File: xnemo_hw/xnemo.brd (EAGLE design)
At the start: 38.6 x 29.8 mm, 34 parts, among them J1 MICRO_USB_B_RECEPT, J2 DM3D_MICRO_SD, J3 HEADER_2X5_0.05_SMD, J4 HEADER_2X5_0.05_THRU, J5 HEADER_2X5_0.05_THRU, U1 LTC3559, U2 L3GD20, U3 STM32F405RG, U5 HMC5883L, U6 ADXL345, X1 TXC_7A_XTAL

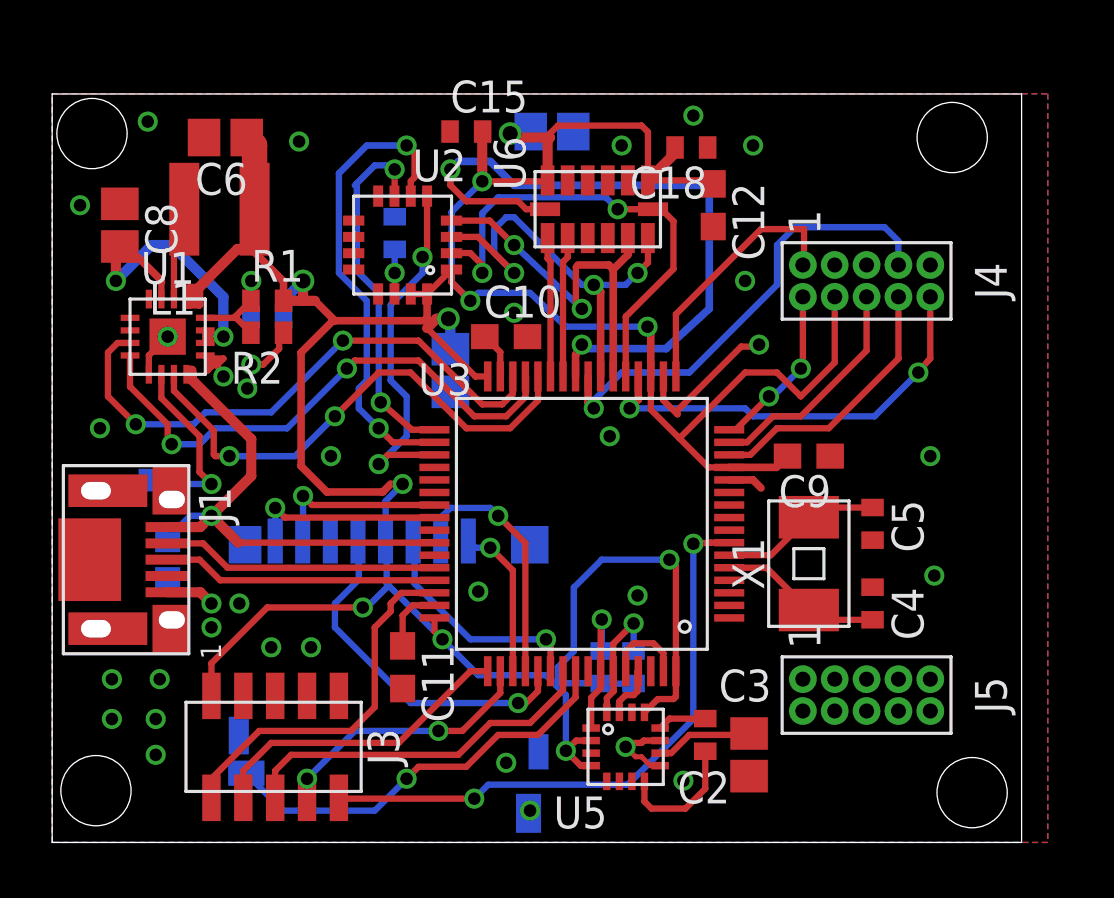
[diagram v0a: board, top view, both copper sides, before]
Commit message: r1 submitted
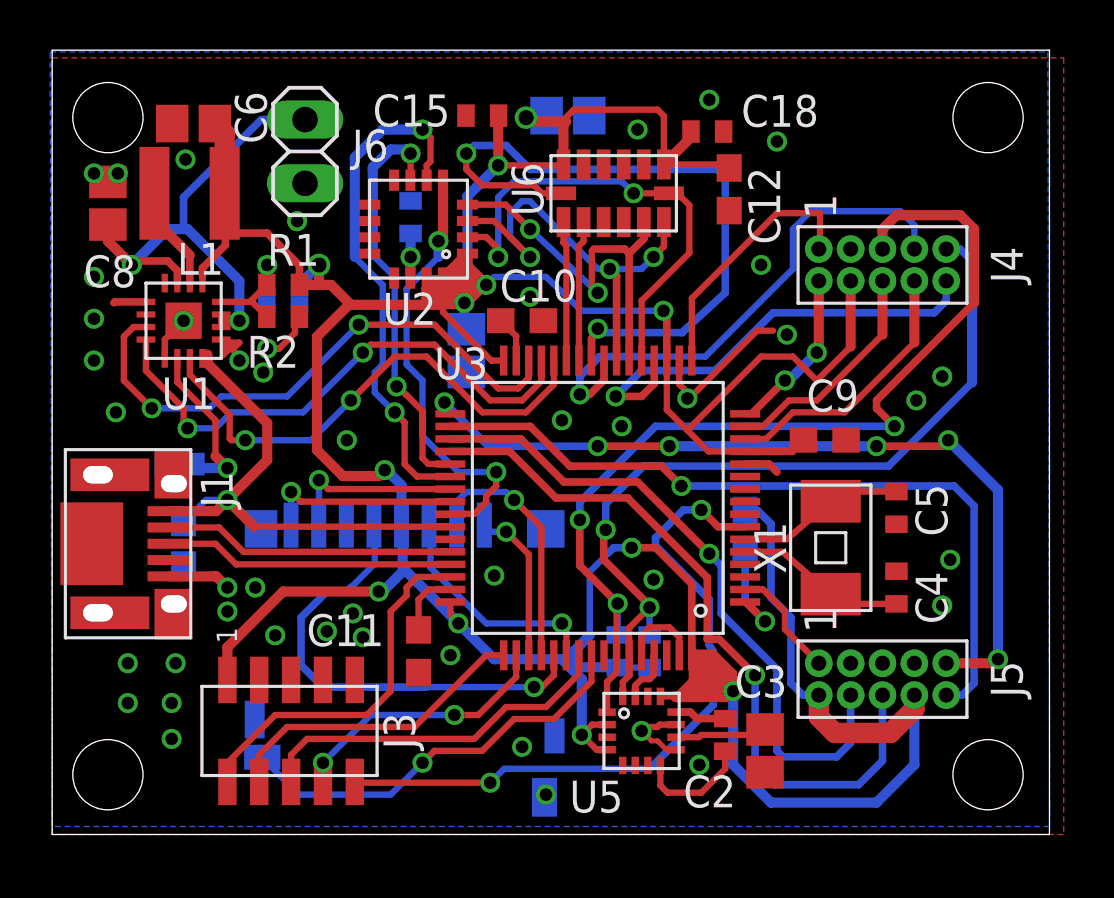
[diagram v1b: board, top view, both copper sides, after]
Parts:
- added C13: 2.2u, resistor:C0603
- added J6: (no value), pinhead:1X02
- moved C6 1.39 mm to (5.64, 28.3)
- moved L1 1.35 mm to (5.48, 25.6)
- moved C4 1.14 mm to (33.7, 9.84)
- moved C5 1.14 mm to (33.7, 13.0)
- moved X1 1.08 mm to (31.0, 11.4)
- moved C16 1.02 mm to (16.5, 19.3)
- moved C8 0.99 mm to (2.22, 25.2)
- moved J4 0.90 mm to (33.1, 22.7)
- moved J5 0.90 mm to (33.1, 6.19)
- moved C10 0.90 mm to (18.7, 20.5)
- moved C12 0.90 mm to (27.0, 25.7)
- moved C17 0.90 mm to (20.6, 28.7)
- moved U5 0.90 mm to (23.5, 4.13)
- moved C14 0.90 mm to (9.21, 21.3)
- moved J2 0.90 mm to (13.3, 6.35)
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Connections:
- removed net N$1: J5.P$4
- removed net N$16: J5.P$7
- removed net N$17: J5.P$5
- removed net N$2: J5.P$2
- removed net N$3: J5.P$3
- removed net N$4: J5.P$1
- removed net N$5: J5.P$6
- removed net N$6: J5.P$8
- removed net N$7: J4.P$9
- removed net N$8: J5.P$10
- removed net N$9: J5.P$9
- new net PA10: U3.P$43
- new net PB12: J5.P$9, U3.P$33
- new net PB13: J5.P$10, U3.P$34
- new net PB14: J5.P$4, U3.P$35
- new net PB15: J5.P$6, U3.P$36
- new net PC13: J5.P$1, U3.P$2
- new net UC_VBAT: C13.2, U3.P$1
- net 3V3: now also C13.1, J5.P$2, J5.P$8
- net GND: now also J5.P$3, J5.P$5, J5.P$7, J6.1
- net GYR_DRDY: now also U3.P$38; no longer U3.P$34
- net GYR_INT1: now also U3.P$37; no longer U3.P$33
- net I2C_SCL: now also J4.P$5
- net I2C_SDA: now also J4.P$9
- net PA1: no longer J4.P$5
- net SPI_CS_GYR: now also U3.P$41; no longer U3.P$35
- net VBAT: now also J6.2
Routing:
- net 3V3: track 144.7 -> 191.3 mm, vias 11 -> 12
- net PB12: track 0.00 -> 33.1 mm, vias 0 -> 6
- net I2C_SCL: track 5.76 -> 38.9 mm, vias 1 -> 3
- net PB13: track 0.00 -> 30.6 mm, vias 0 -> 1
- net PB15: track 0.00 -> 29.3 mm, vias 0 -> 1
- net I2C_SDA: track 5.10 -> 32.7 mm, vias 1 -> 2
- net PB14: track 0.00 -> 26.4 mm, vias 0 -> 1
- net VBAT: track 13.6 -> 20.6 mm
- net PC13: track 0.00 -> 4.57 mm
- net SD_CLK: track 14.2 -> 18.7 mm
- net UC_VBAT: track 0.00 -> 4.19 mm, vias 0 -> 1
- net RESET: track 23.9 -> 27.5 mm
- net SPI_CS_GYR: track 14.4 -> 17.6 mm
- net PC4: track 18.8 -> 20.9 mm
- net GND: track 22.9 -> 24.8 mm, vias 34 -> 45
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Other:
- board size 38.6 x 29.8 mm -> 39.8 x 31.3 mm
- board text added: "bnahill@gmail.com"
- board text added: "xNEMO r1"
